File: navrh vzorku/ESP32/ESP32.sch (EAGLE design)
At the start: 19 parts, among them U1 ESP-WROOM-32

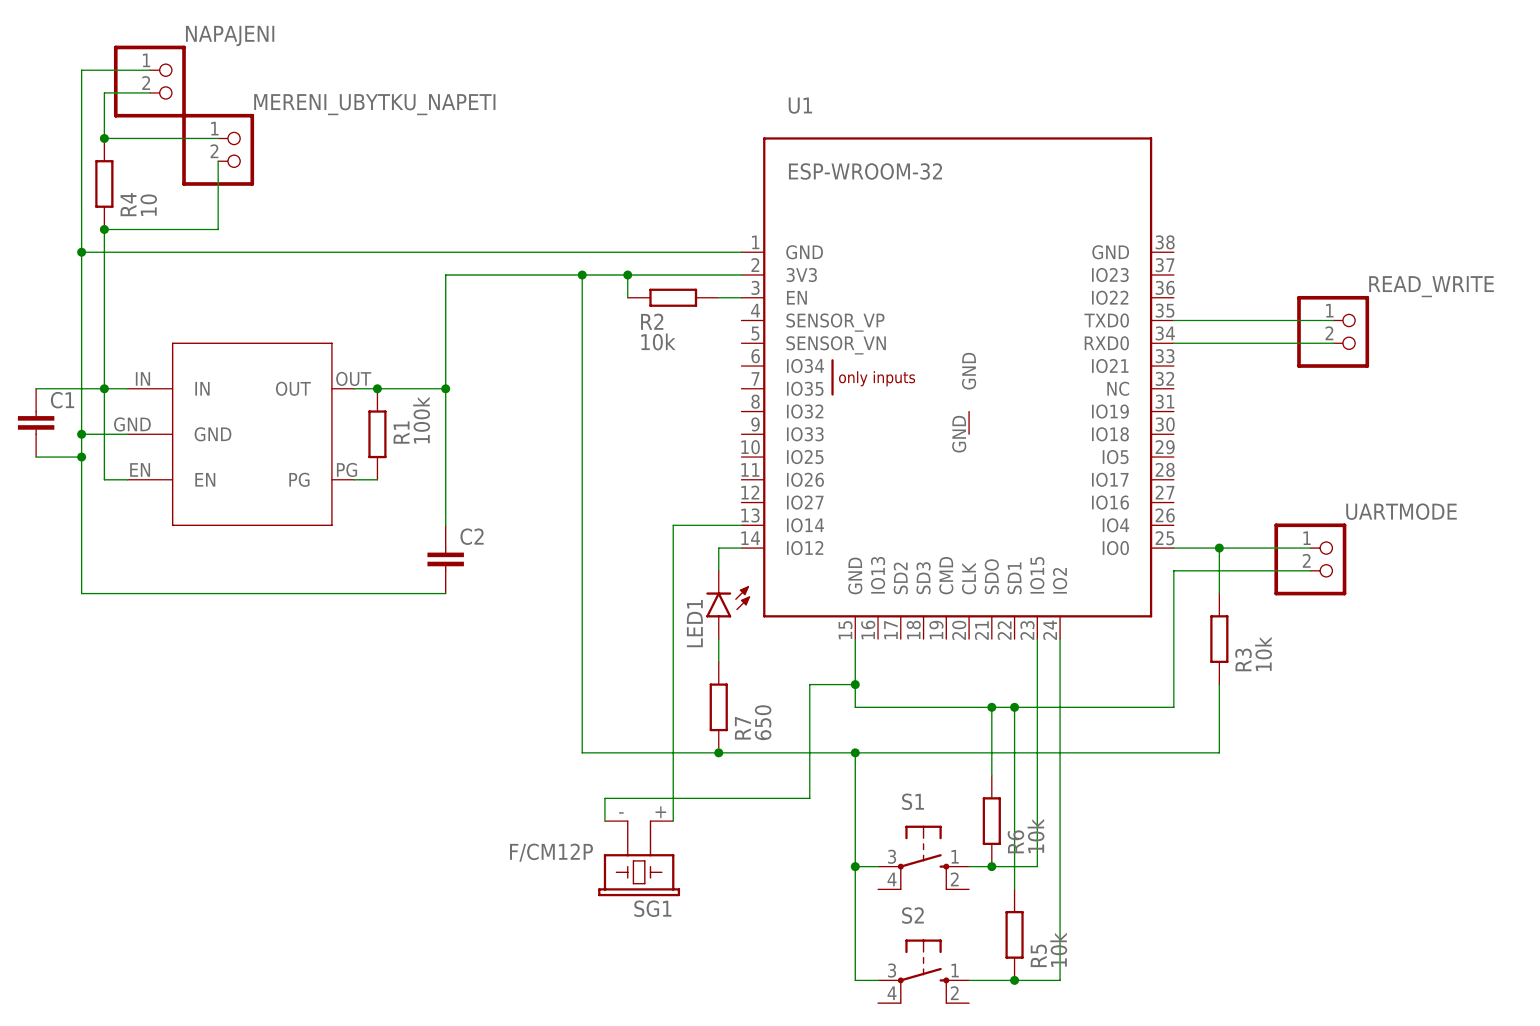
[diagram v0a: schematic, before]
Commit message: Program funčního vzorku ESP
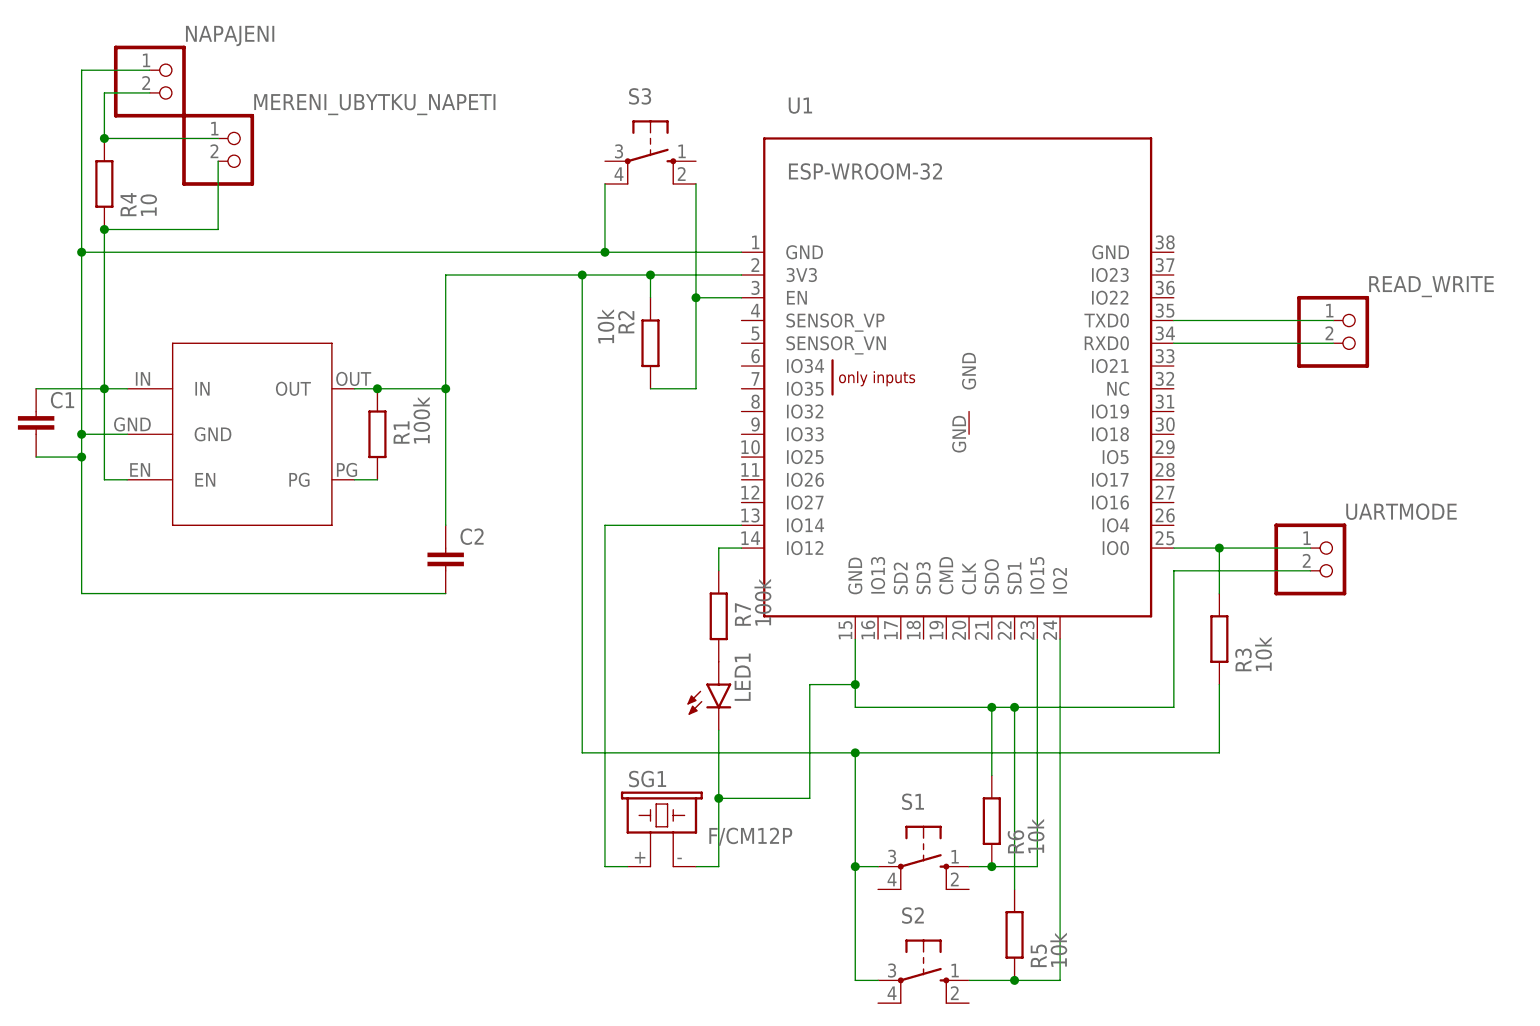
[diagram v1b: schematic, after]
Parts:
- added S3: (no value), switch-omron:10-XX
- R7: value 650 -> 100k
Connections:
- removed net N$15: LED1.A, R7.2
- new net N$9: R7.2, U1.IO12
- net N$14: now also LED1.A, R7.1; no longer LED1.C, U1.IO12
- net N$16: now also LED1.C
- net N$2: no longer R7.1
- net N$3: now also S3.P1
- net N$5: now also S3.S1
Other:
- moved on the sheet: LED1, R2, R7, SG1
